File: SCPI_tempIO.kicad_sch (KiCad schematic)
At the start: 19 parts, among them J1 Conn_ARM_JTAG_SWD_10, J2 Conn_02x05_Odd_Even, P1 USB_C_Plug_USB2.0, SW1 SW_SPST, U1 STM32G070KBTx, U2 AP2112K-3.3, U3 SHT4x

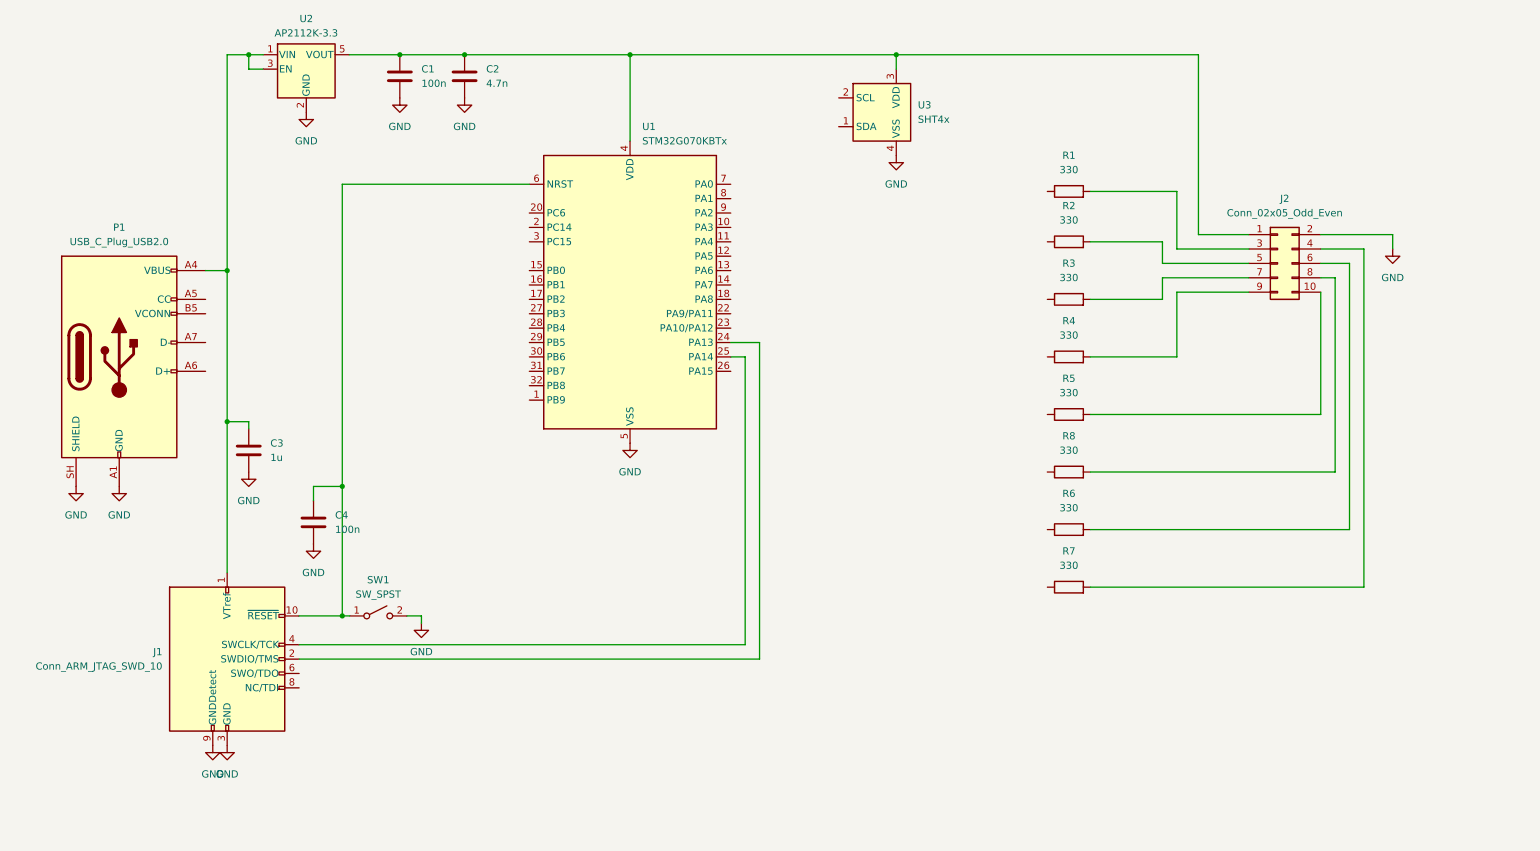
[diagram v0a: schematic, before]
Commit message: USB for contemporary goodness
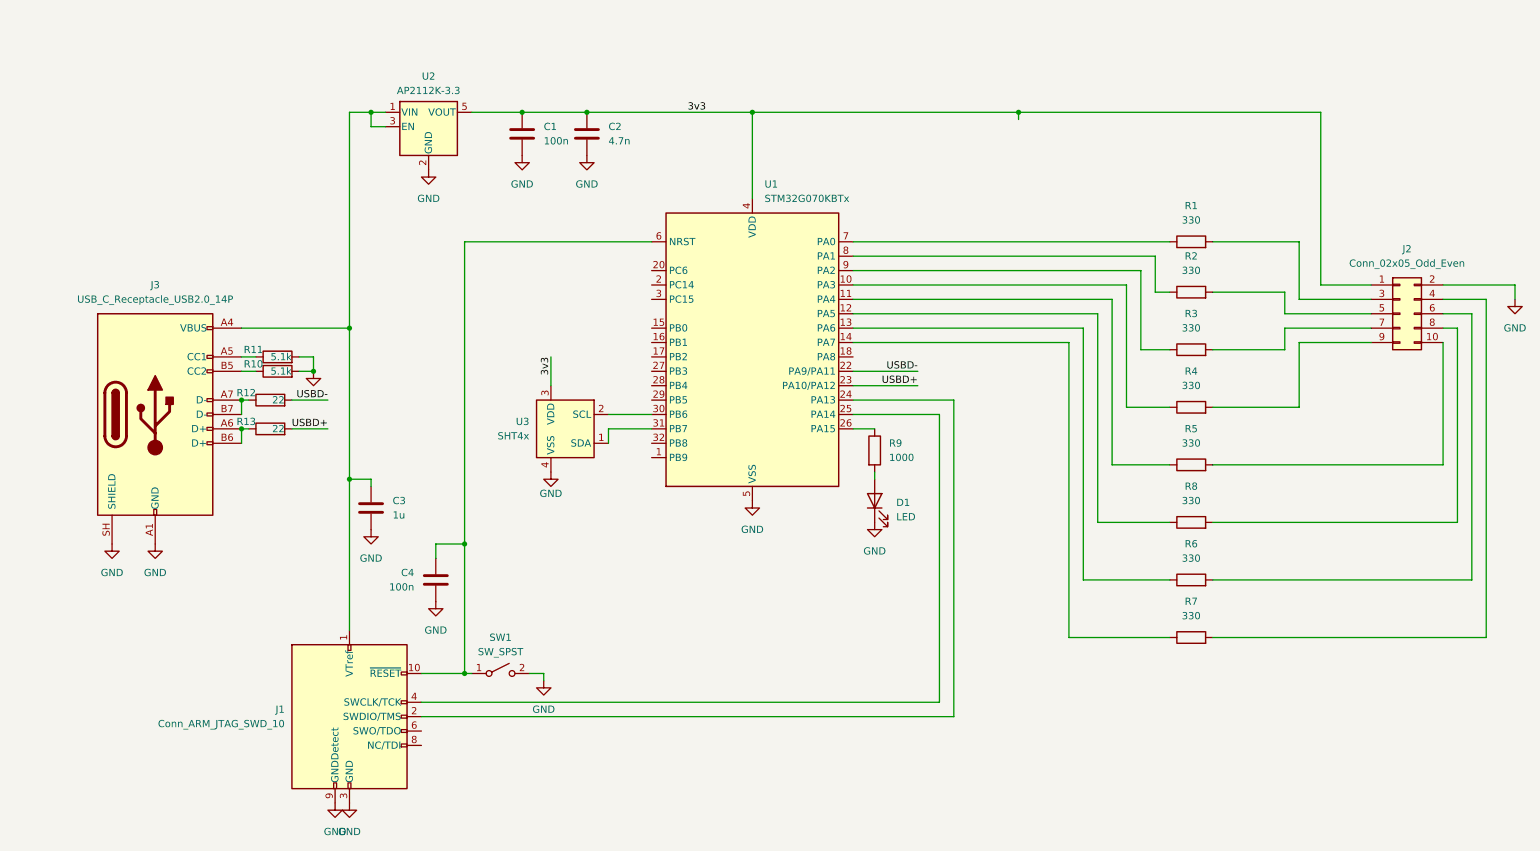
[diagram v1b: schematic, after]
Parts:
- removed P1: USB_C_Plug_USB2.0, symbol Connector:USB_C_Plug_USB2.0
- added D1: LED, LED_SMD:LED_01005_0402Metric_Pad0.57x0.30mm_HandSolder, symbol Device:LED
- added J3: USB_C_Receptacle_USB2.0_14P, symbol Connector:USB_C_Receptacle_USB2.0_14P
- added R10, R11: 5.1k, Resistor_SMD:R_0402_1005Metric, symbol Device:R
- added R12, R13: 22, Resistor_SMD:R_0402_1005Metric, symbol Device:R
- added R9: 1000, Resistor_SMD:R_0402_1005Metric, symbol Device:R
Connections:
- net GND: now also D1.1 (K), J3.A1 (GND), J3.A12 (GND), J3.B1 (GND), J3.B12 (GND), J3.SH (SHIELD), R10.2, R11.2
- net at R6.1: now also U1.13 (PA6)
- net at R4.1: now also U1.10 (PA3)
- net 3v3: now reaches C1.1, C2.1, J2.1 (Pin_1), U1.4 (VDD), U2.5 (VOUT), U3.3 (VDD)
- net at R2.1: now also U1.8 (PA1)
- net at U1.11 (PA4): now also R5.1
- net at U1.12 (PA5): now also R8.1
- net at U1.14 (PA7): now also R7.1
- net USBD-: now reaches U1.22 (PA9/PA11)
- net USBD-: now also R12.2
- net USBD+: now reaches U1.23 (PA10/PA12)
- net USBD+: now also R13.2
- net at U1.26 (PA15): now also R9.1
- net at U1.30 (PB6): now also U3.2 (SCL)
- net at U1.31 (PB7): now also U3.1 (SDA)
- net at U1.7 (PA0): now also R1.1
- net at U1.9 (PA2): now also R3.1
- net at C3.1, J1.1 (VTref), U2.1 (VIN)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: now also J3.A4 (VBUS), J3.A9 (VBUS), J3.B4 (VBUS), J3.B9 (VBUS)
- new net: J3.B5 (CC2), R10.1
- new net: J3.A7 (D-), J3.B7 (D-), R12.1
- new net: J3.A5 (CC1), R11.1
- new net: J3.A6 (D+), J3.B6 (D+), R13.1
- new net: D1.2 (A), R9.2
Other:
- moved on the sheet: C1, C2, C3, C4, J1, J2, R1, R2, R3, R4, R5, R6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
